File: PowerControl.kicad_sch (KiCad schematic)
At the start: 49 parts, among them J1 INPUT_JACK, Q1 KT315D, Q13 KT315, Q2 KT315D, Q3 2n3906, Q4 2n3906, Q7 2n3904, Q8 2n3904, Q9 JE350, U8 MC33063AP

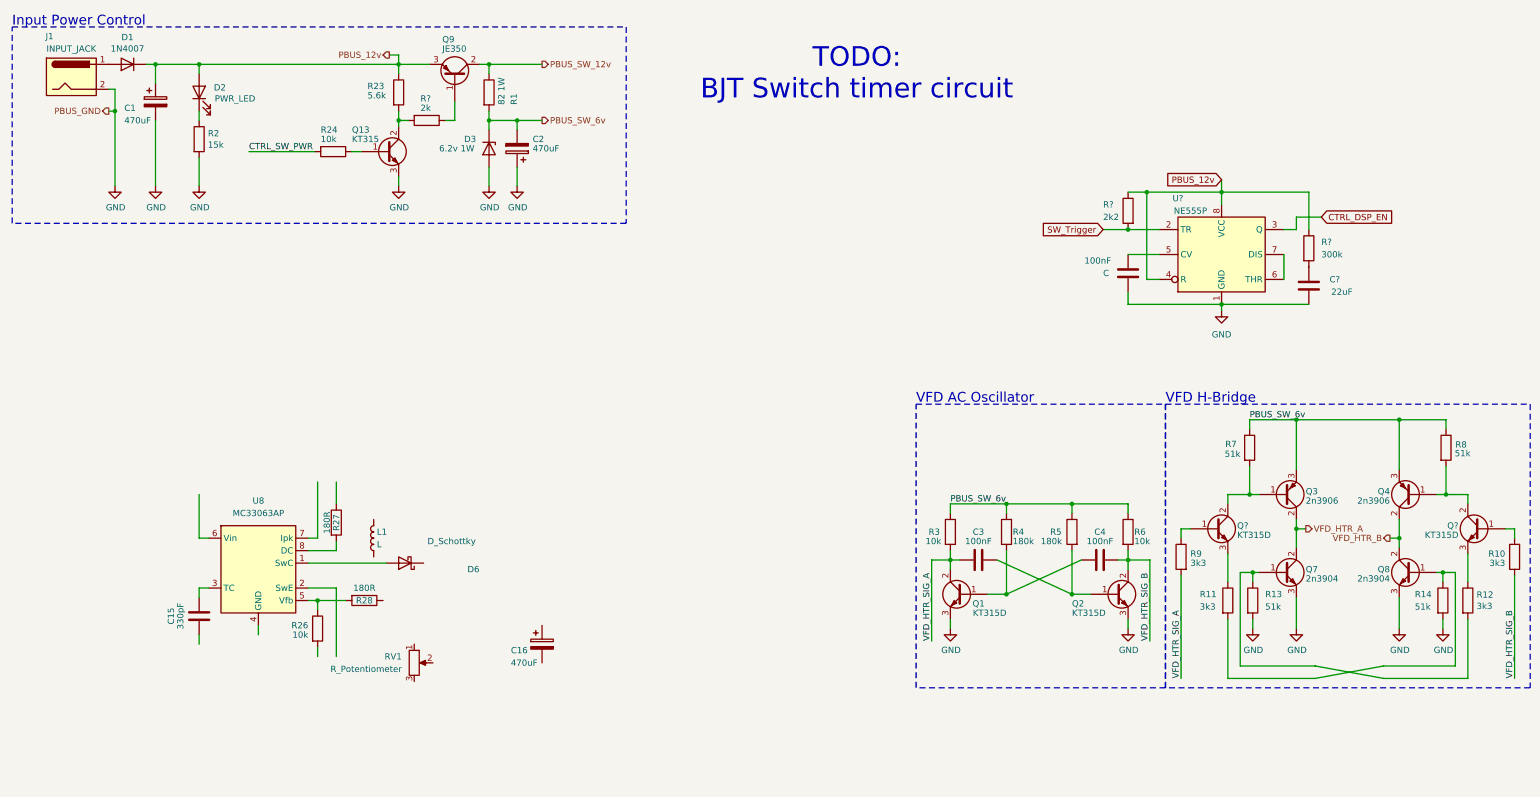
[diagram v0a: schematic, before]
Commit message: PSU Schematic Finished
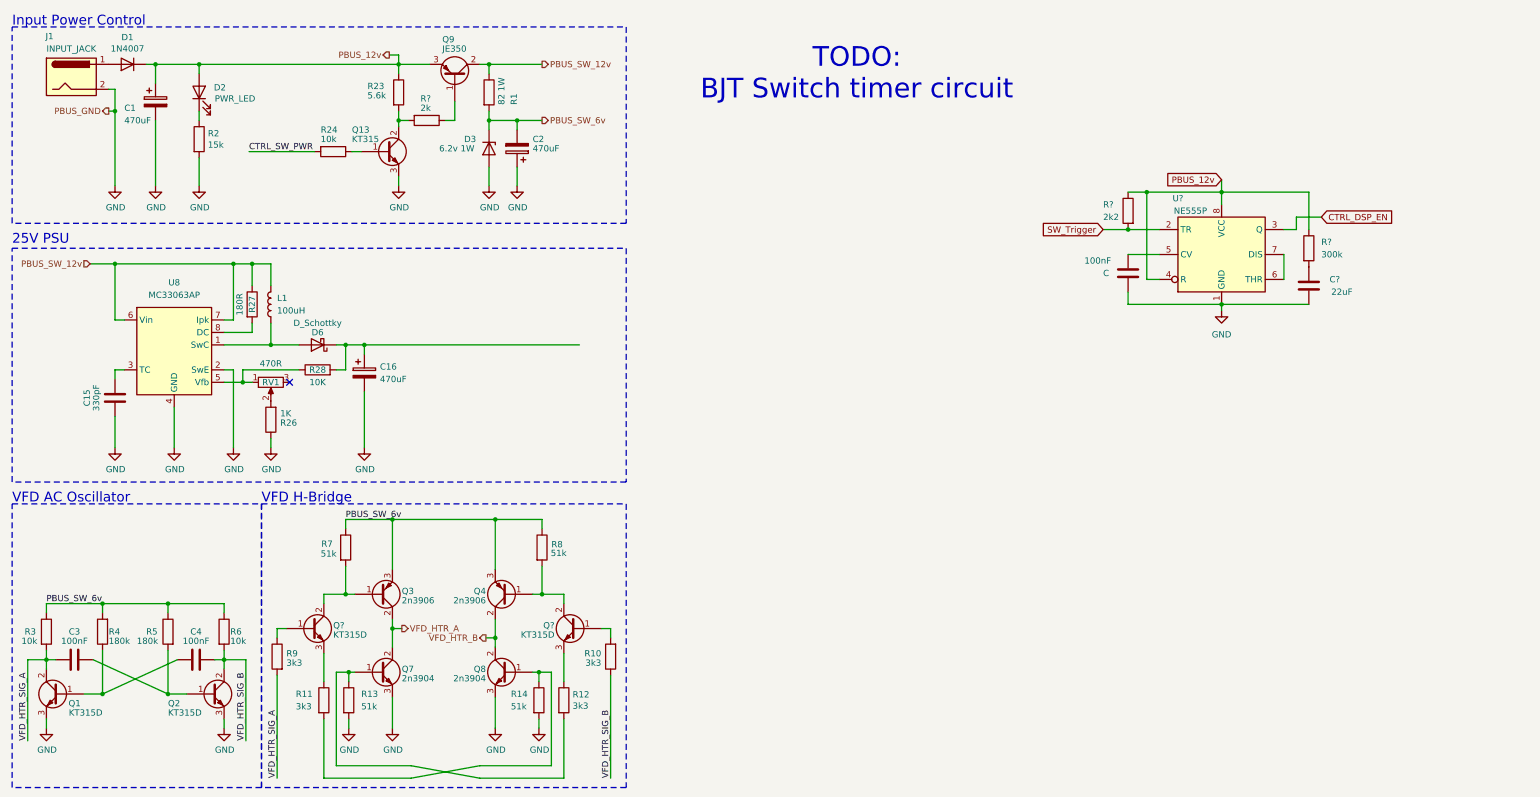
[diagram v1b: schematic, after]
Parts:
- L1: value L -> 100uH
- R26: value 10k -> 1K
- R28: value 180R -> 10K
- RV1: value R_Potentiometer -> 470R
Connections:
- net GND: now also C15.2, C16.2, R26.1, U8.2 (SwE), U8.4 (GND)
- net PBUS_SW_12v: now also L1.2, R27.1, U8.6 (Vin), U8.7 (Ipk)
- net at RV1.1: now also R28.1, U8.5 (Vfb)
- net at RV1.2: now also R26.2
- net at L1.1: now also D6.2 (A), U8.1 (SwC)
- net at D6.1 (K): now also C16.1, R28.2
- no-connect marks 0 -> 1
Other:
- note added: "25V PSU"
- moved on the sheet: C15, C16, C3, C4, D6, L1, Q1, Q2, Q3, Q4, Q7, Q8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
